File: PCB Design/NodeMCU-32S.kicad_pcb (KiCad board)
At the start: 2 copper layers, 85.4 x 61.5 mm, 18 parts, among them J1 Screw_Terminal_01x02, J2 Screw_Terminal_01x02, J3 Screw_Terminal_01x04, J5 Screw_Terminal_01x03, Q1 IRLZ44N, SW1 SW_DPDT_x2, U1 ESP32-DevKitC, U2 Generic_5v_Module

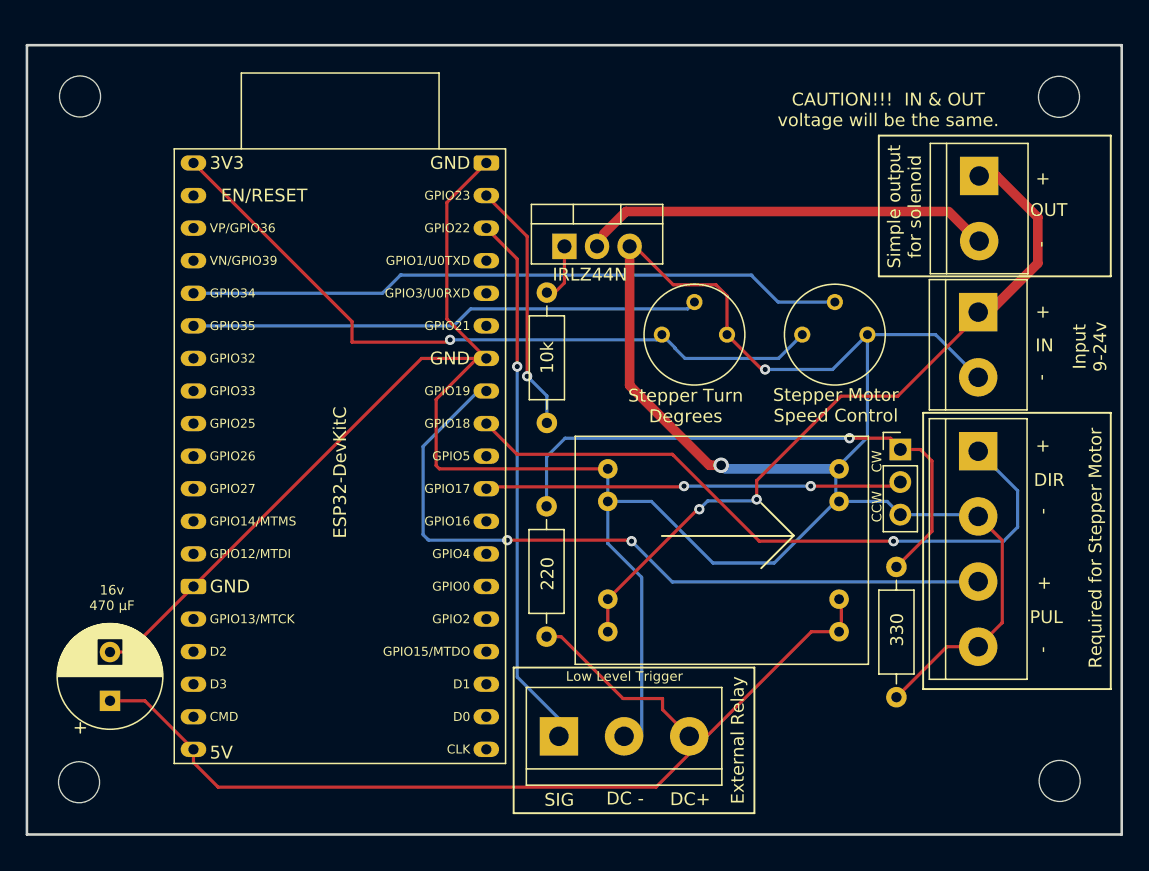
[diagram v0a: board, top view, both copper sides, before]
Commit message: Cleanerer
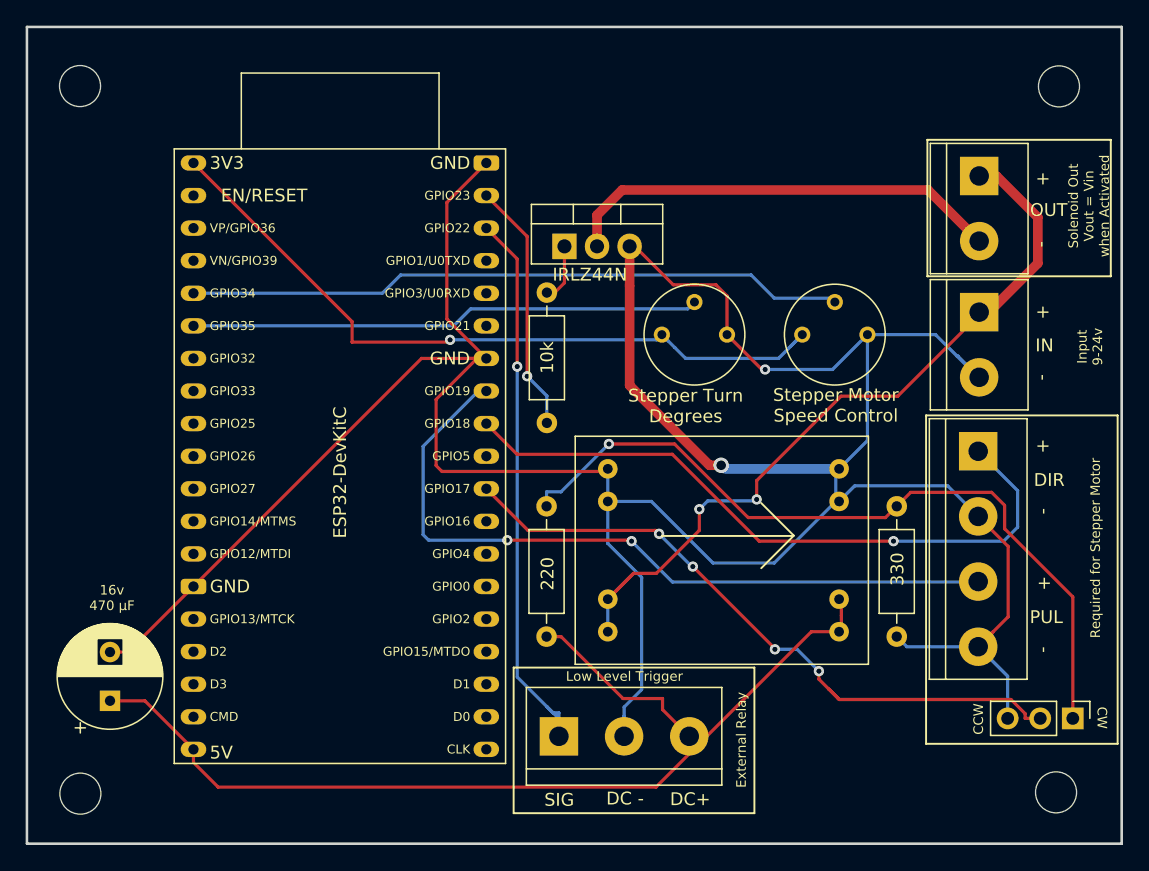
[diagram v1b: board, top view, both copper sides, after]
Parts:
- moved SW1 24.9 mm to (141.0, 104.3), turned to -90 degrees
- moved R4 4.72 mm to (127.2, 87.7)
- moved H1 0.93 mm to (139.6, 110.0)
- moved H3 0.89 mm to (63.6, 110.1)
- moved H4 0.81 mm to (139.9, 55.0)
- moved H2 0.81 mm to (63.6, 55.0)
- moved J2 0.08 mm to (133.7, 72.6)
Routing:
- net Net-(SW1-Pad2): track 32.6 -> 52.3 mm, vias 2 -> 4
- net Net-(R3-Pad2): track 44.7 -> 60.8 mm
- net GND: track 234.3 -> 247.9 mm
- net MOSFET_GND: track 31.5 -> 35.6 mm
- net VCC: track 56.7 -> 60.1 mm
- net +5V: track 82.7 -> 80.5 mm
- net lowActivationPin: track 42.5 -> 44.2 mm
- net Net-(Q1-Pad1): track 3.96 -> 3.25 mm
- net PUL: track 58.4 -> 57.8 mm
- net +3V3: track 56.0 -> 56.6 mm
- net SPEED_POT: track 51.5 -> 51.0 mm
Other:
- board size 85.4 x 61.5 mm -> 85.4 x 63.7 mm
- board text added: "Board Design 1.7"
- board text added: "Solenoid Out Vout = Vin when Activated"
- board text removed: "Board Design 1.6"
- board text removed: "CAUTION!!! IN & OUT voltage will be the same."
- board text removed: "Simple output for solenoid"
